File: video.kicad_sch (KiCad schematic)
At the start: 29 parts, among them J3 Conn_02x16_Odd_Even

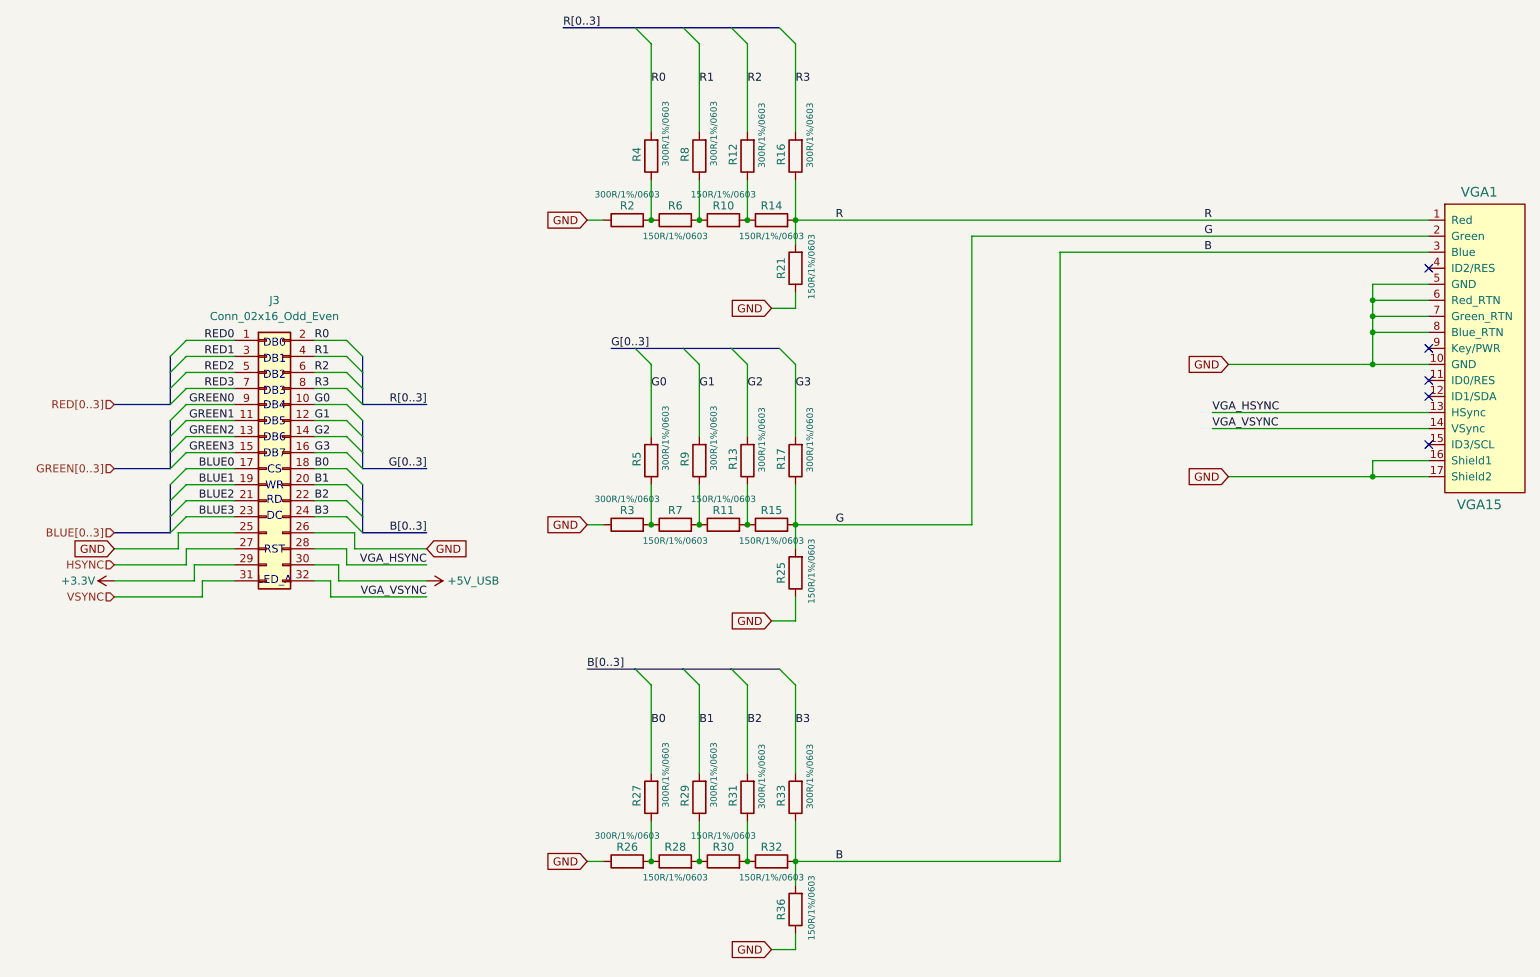
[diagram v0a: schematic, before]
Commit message: 1st production and BOM
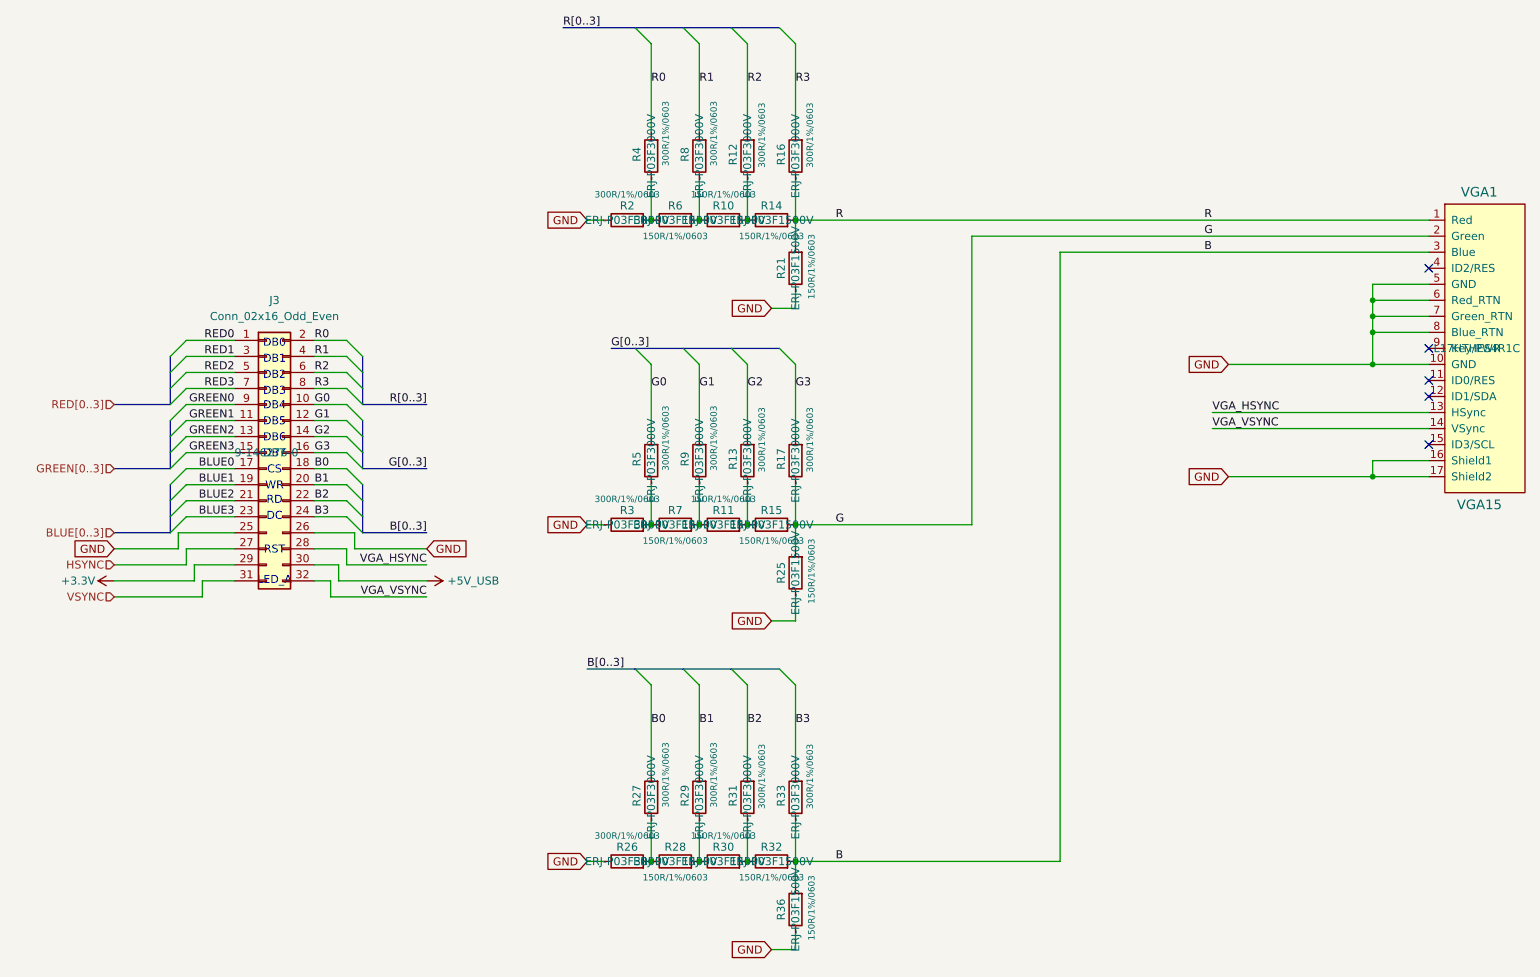
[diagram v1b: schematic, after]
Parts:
- J3: MfgNumber (none) -> 9-146276-0
- R10, R11, R14, R15, R21, R25, R28, R30, R32, R36, R6, R7: MfgNumber (none) -> ERJ-P03F1500V
- R12, R13, R16, R17, R2, R26, R27, R29, R3, R31, R33, R4, R5, R8, R9: MfgNumber (none) -> ERJ-P03F3000V
- VGA1: MfgNumber (none) -> L17HTHES4R1C
